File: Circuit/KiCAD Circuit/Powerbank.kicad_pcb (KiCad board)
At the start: 2 copper layers, 96.5 x 99.1 mm, 44 parts, among them J1 EBWA-04-A, Q1 NMOS, Q2 PMOS, Q3 NMOS, SW1 SW_Push, SW2 SW_SPST, U1 BQ7692003PW

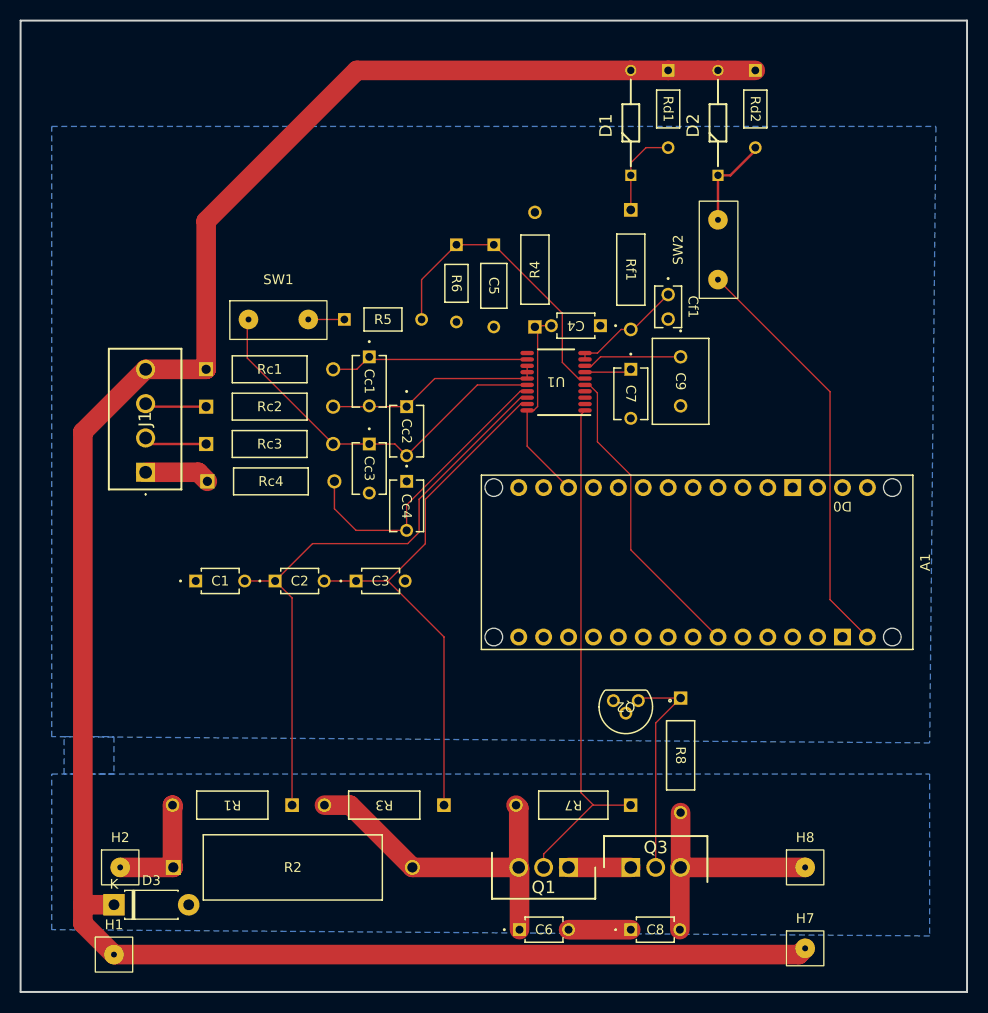
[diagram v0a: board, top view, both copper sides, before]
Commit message: Backup
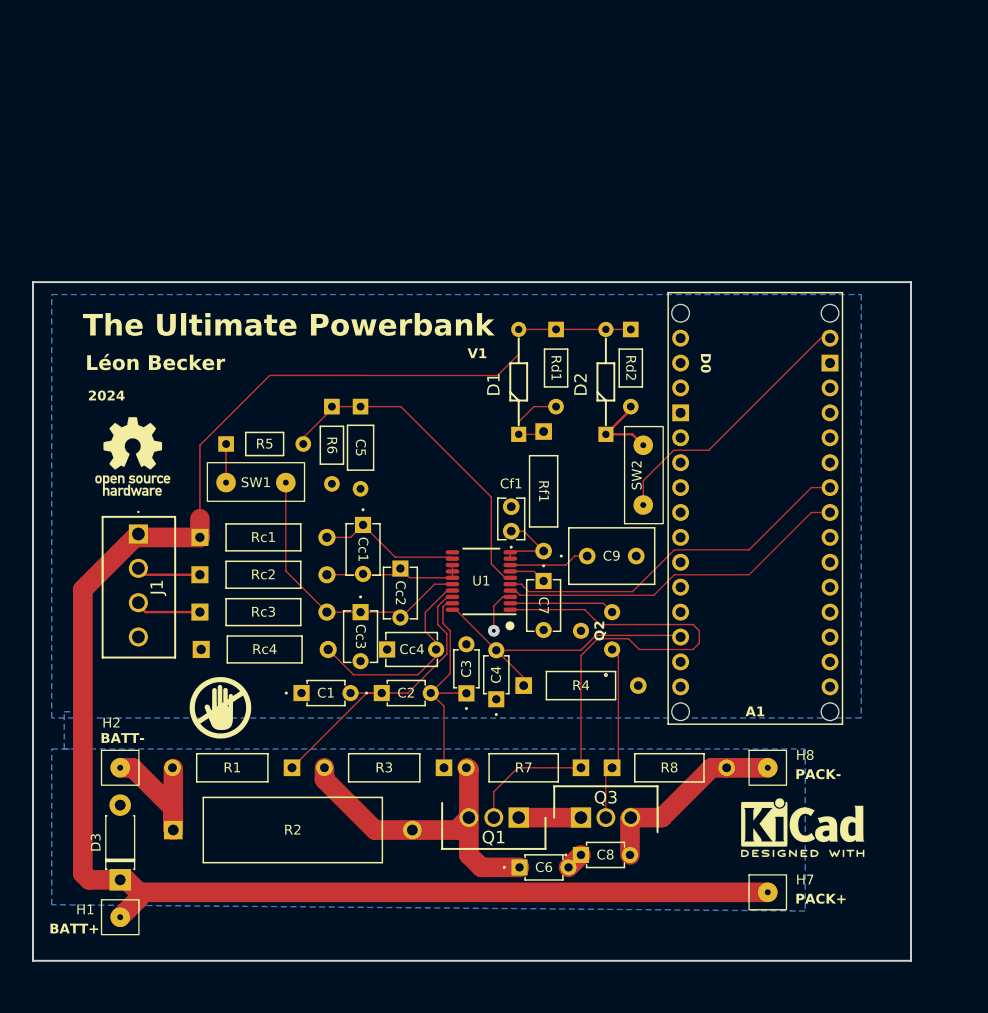
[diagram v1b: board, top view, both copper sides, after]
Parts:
- added G1: LOGO, Symbol:Do Not Touch Symbol, F.Cu at (111.8, 118.4)
- added G2: OSHW-Logo_7.5x8mm_SilkScreen, Symbol:OSHW-Logo_7.5x8mm_SilkScreen, F.Cu at (102.9, 92.7)
- added NT1: NetTie, Custom Footprints:NetTie General Net Class, F.Cu at (109.7, 97.8)
- added NT2: NetTie, Custom Footprints:NetTie General Net Class, F.Cu at (139.7, 109.2)
- added REF1: KiCad-Logo2_5mm_SilkScreen, Symbol:KiCad-Logo2_5mm_SilkScreen, F.Cu at (171.2, 130.6)
- Q2: footprint VP3203N3-G:TO-92_MC_MCH -> Custom Footprints:TO-92_MC_MCH
- moved C4 39.6 mm to (140.0, 117.5), turned to 90 degrees
- moved R4 36.6 mm to (142.7, 116.1), turned to 0 degrees
- moved A1 32.5 mm to (166.4, 120.0), turned to 0 degrees
- moved Rd2 29.3 mm to (153.7, 79.8)
- moved Cf1 29.0 mm to (141.5, 100.3), turned to 90 degrees
- moved D2 28.8 mm to (151.1, 85.4)
- moved D1 28.8 mm to (142.2, 85.4)
- moved Rd1 28.8 mm to (146.1, 79.8)
- moved Rf1 24.3 mm to (144.8, 90.2)
- moved SW2 24.2 mm to (154.9, 94.6)
- moved C7 23.3 mm to (144.8, 105.4)
- moved C9 22.4 mm to (149.2, 102.9), turned to 0 degrees
- moved U1 21.7 mm to (138.4, 105.4)
- moved C5 21.4 mm to (126.1, 87.6)
- moved R6 20.8 mm to (123.2, 87.6)
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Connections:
- D3 pad 1: Net-(D1-A) -> Net-(D3-K)
- H1 pad 1: Net-(D1-A) -> Net-(D3-K)
- H7 pad 1: Net-(D1-A) -> Net-(D3-K)
- J1 pad 4: Net-(D1-A) -> Net-(D3-K)
- Rc1 pad 1: Net-(D1-A) -> Net-(D3-K)
- U1 pad 3: GND -> Net-(U1-VSS)
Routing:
- net Net-(D1-A): track 221.2 -> 55.3 mm
- net Net-(D3-K): track 0.00 -> 119.5 mm
- net Net-(A1-A4/SDA): track 0.00 -> 37.0 mm
- net Net-(U1-SRN): track 56.0 -> 22.9 mm
- net Net-(U1-SRP): track 62.1 -> 30.9 mm
- net Net-(SW2-A): track 42.8 -> 27.5 mm
- net Net-(Q2-S): track 0.00 -> 10.8 mm
- net Net-(U1-VC1): track 39.6 -> 29.4 mm
- net Net-(U1-ALERT): track 21.3 -> 31.3 mm
- net Net-(U1-VC0): track 30.8 -> 22.1 mm
- net Net-(U1-VC2): track 22.3 -> 14.8 mm
- net Net-(A1-A5/SCL): track 31.6 -> 37.3 mm
- net Net-(U1-VC5): track 20.4 -> 14.7 mm
- net Net-(Q1-G): track 53.2 -> 58.9 mm
- net Net-(U1-TS1): track 30.8 -> 35.7 mm
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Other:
- board size 96.5 x 99.1 mm -> 89.5 x 69.2 mm
- board text added: "2024"
- board text added: "BATT+"
- board text added: "BATT-"
- board text added: "Léon Becker"
- board text added: "PACK+"
- board text added: "PACK-"
- board text added: "The Ultimate Powerbank"
- board text added: "V1"

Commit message: Backup
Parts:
- C1, C2, C3, C6, C8: value 0.1μF -> 0.1uF
- C7, Cc1, Cc2, Cc3, Cc4: value 1μF -> 1uF
- C9: value 4.7μF -> 4.7uF
- Cf1: value 2.2μF -> 2.2uF
- R1, R3, Rf1: value 100Ω -> 100
- R2: value 8mΩ -> 8m
- R4: value 499kΩ -> 499k
- R5, R6, Rd1, Rd2: value 10kΩ -> 10k
- R7, R8: value 1MΩ -> 1M
- Rc1, Rc2, Rc3, Rc4: value 50Ω -> 50
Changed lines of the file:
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@@
 			)
 		)
-		(property "Value" "2.2μF"
+		(property "Value" "2.2uF"
 			(at 1.25 0 90)
 			(unlocked yes)
@@
 			)
 		)
-		(property "Value" "1MΩ"
+		(property "Value" "1M"
 			(at 5.842 0 0)
 			(unlocked yes)
@@
 		(fp_arc
 			(start 2.199991 3.050012)
-			(mid 2.141408 3.191422)
+			(mid 2.141406 3.191427)
 			(end 1.999991 3.250011)
 			(stroke
@@
 			)
 		)
-		(property "Value" "100Ω"
+		(property "Value" "100"
 			(at 6.096 0 180)
 			(unlocked yes)
@@
 			)
 		)
-		(property "Value" "1μF"
+		(property "Value" "1uF"
 			(at 2.5 0 -90)
 			(unlocked yes)
@@
 			)
 		)
-		(property "Value" "50Ω"
+		(property "Value" "50"
 			(at 6.477 0 0)
 			(unlocked yes)
@@
 			)
 		)
-		(property "Value" "499kΩ"
+		(property "Value" "499k"
 			(at 5.842 0 0)
 			(unlocked yes)
@@
 		)
 		(property "Mouser" "603-MFR-25FBF52-499K"
-			(at 0 0 360)
+			(at 0 0 0)
 			(layer "F.Fab")
 			(hide yes)
@@
 			)
 		)
-		(property "Value" "10kΩ"
+		(property "Value" "10k"
 			(at 3.937 0 0)
 			(unlocked yes)
@@
 			)
 		)
-		(property "Value" "50Ω"
+		(property "Value" "50"
 			(at 6.477 0 0)
 			(unlocked yes)
@@
 			)
 		)
-		(property "Value" "4.7μF"
+		(property "Value" "4.7uF"
 			(at 2.5 0 0)
 			(unlocked yes)
@@
 			)
 		)
-		(property "Value" "0.1μF"
+		(property "Value" "0.1uF"
 			(at 2.499995 0 0)
 			(unlocked yes)
@@
 			)
 		)
-		(property "Value" "1MΩ"
+		(property "Value" "1M"
 			(at 5.842 0 180)
 			(unlocked yes)
@@
 		(tags "Logo KiCad")
 		(property "Reference" "REF1"
-			(at 0 -5.08 360)
+			(at 0 -5.08 0)
 			(layer "F.SilkS")
 			(hide yes)
@@
 		)
 		(property "Value" "KiCad-Logo2_5mm_SilkScreen"
-			(at 0 5.08 360)
+			(at 0 5.08 0)
 			(layer "F.Fab")
 			(hide yes)
@@
 		)
 		(property "Mouser" "594-K471K10X7RF5UH5"
-			(at 0 0 270)
+			(at 0 0 -90)
 			(layer "F.Fab")
 			(hide yes)
@@
 			)
 		)
-		(property "Value" "10kΩ"
+		(property "Value" "10k"
 			(at 3.937 0 -90)
 			(unlocked yes)
@@
 			)
 		)
-		(property "Value" "1μF"
+		(property "Value" "1uF"
 			(at 2.5 0 -90)
 			(unlocked yes)
@@
 			)
 		)
-		(property "Value" "1μF"
+		(property "Value" "1uF"
 			(at 2.5 0 0)
 			(unlocked yes)
@@
 			)
 		)
+		(property ki_fp_filters "C_*")
+		(sheetname "Root")
+		(sheetfile "Powerbank.kicad_sch")
 		(attr through_hole)
 		(fp_line
@@
 			)
 		)
-		(property "Value" "10kΩ"
+		(property "Value" "10k"
 			(at 3.937 0 -90)
 			(unlocked yes)
@@
 			)
 		)
-		(property "Value" "100Ω"
+		(property "Value" "100"
 			(at 6.096 0 180)
 			(unlocked yes)
@@
 			)
 		)
-		(property "Value" "8mΩ"
+		(property "Value" "8m"
 			(at 12.192 0 0)
 			(unlocked yes)
@@
 			)
 		)
-		(property "Value" "0.1μF"
+		(property "Value" "0.1uF"
 			(at 2.499995 0 0)
 			(unlocked yes)
@@
 			)
 		)
-		(property "Value" "50Ω"
+		(property "Value" "50"
 			(at 6.477 0 0)
 			(unlocked yes)
@@
 			)
 		)
-		(property "Value" "10kΩ"
+		(property "Value" "10k"
 			(at 3.937 0 -90)
 			(unlocked yes)
@@
 			)
 		)
-		(property "Value" "50Ω"
+		(property "Value" "50"
 			(at 6.477 0 0)
 			(unlocked yes)
@@
 			)
 		)
-		(property "Value" "1μF"
+		(property "Value" "1uF"
 			(at 2.5 0 -90)
 			(unlocked yes)
@@
 			)
 		)
+		(property ki_fp_filters "C_*")
+		(sheetname "Root")
+		(sheetfile "Powerbank.kicad_sch")
 		(attr through_hole)
 		(fp_line
@@
 			)
 		)
-		(property "Value" "0.1μF"
+		(property "Value" "0.1uF"
 			(at 2.499995 0 0)
 			(unlocked yes)
@@
 			)
 		)
-		(property "Value" "0.1μF"
+		(property "Value" "0.1uF"
 			(at 2.499995 0 0)
 			(unlocked yes)
@@
 			)
 		)
-		(property "Value" "100Ω"
+		(property "Value" "100"
 			(at 6.096 0 -90)
 			(unlocked yes)
@@
 			)
 		)
-		(property "Value" "0.1μF"
+		(property "Value" "0.1uF"
 			(at 2.499995 0 90)
 			(unlocked yes)
@@
 		)
 		(property "Mouser" "594-K104K10X7RF53H5"
-			(at 0 0 270)
+			(at 0 0 -90)
 			(layer "F.Fab")
 			(hide yes)
@@
 			)
 		)
-		(property "Value" "1μF"
+		(property "Value" "1uF"
 			(at 2.5 0 -90)
 			(unlocked yes)
